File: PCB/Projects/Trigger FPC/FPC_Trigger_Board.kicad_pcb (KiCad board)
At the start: 2 copper layers, 74.6 x 20.8 mm, 10 parts, among them J1 Conn_01x05_Pin, J2 Conn_01x05_Pin, U1 HAL4395, U2 HAL4395, U3 HAL4395, U4 HAL4395

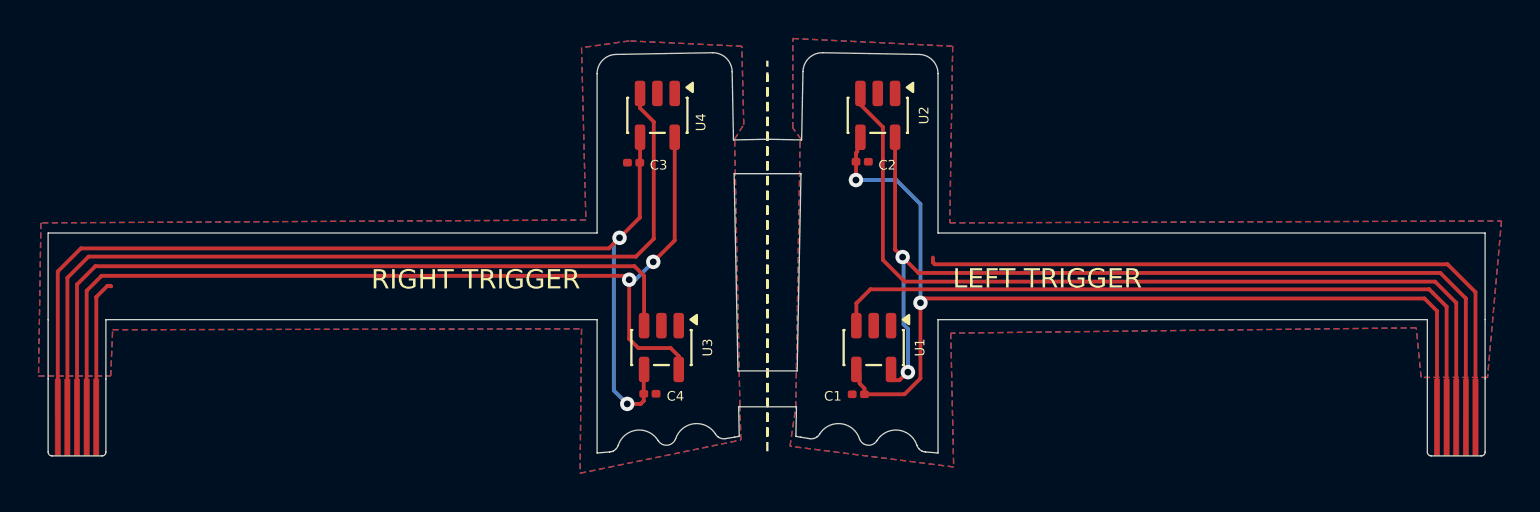
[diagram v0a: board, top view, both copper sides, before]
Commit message: Trigger flex
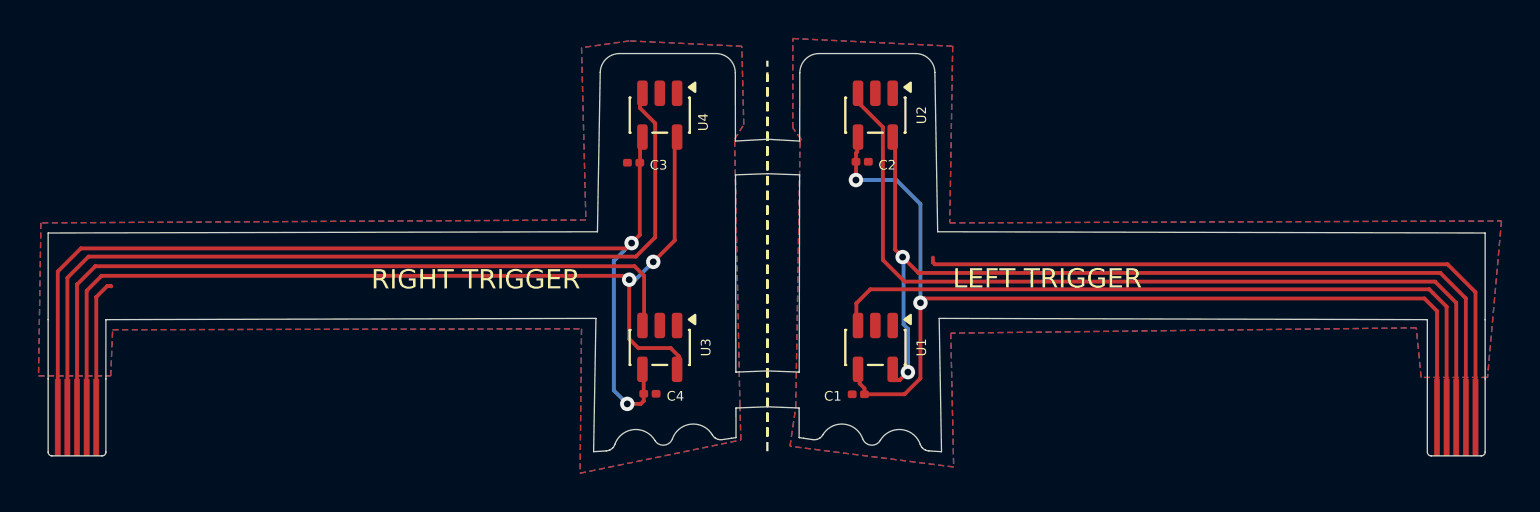
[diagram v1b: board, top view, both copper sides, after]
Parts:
- moved U4 0.13 mm to (230.2, 144.9)
- moved U2 0.13 mm to (241.4, 144.9)
- moved U1 0.09 mm to (241.4, 157.0)
- moved U3 0.09 mm to (230.2, 157.0)
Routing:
- net +3V3: track 54.7 -> 55.2 mm
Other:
- board size 74.6 x 20.8 mm -> 74.6 x 20.7 mm
